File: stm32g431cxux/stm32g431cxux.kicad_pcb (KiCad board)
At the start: 2 copper layers, 17.8 x 31.2 mm, 23 parts, among them J1 USB2.0_C_v3, J2 ProMicro-LeftPin-NoGND, J3 ProMicro-RightPin, SW1 SW_Push, U1 AMS1117-3.3, U2 STM32G431CBUx, Y1 24M

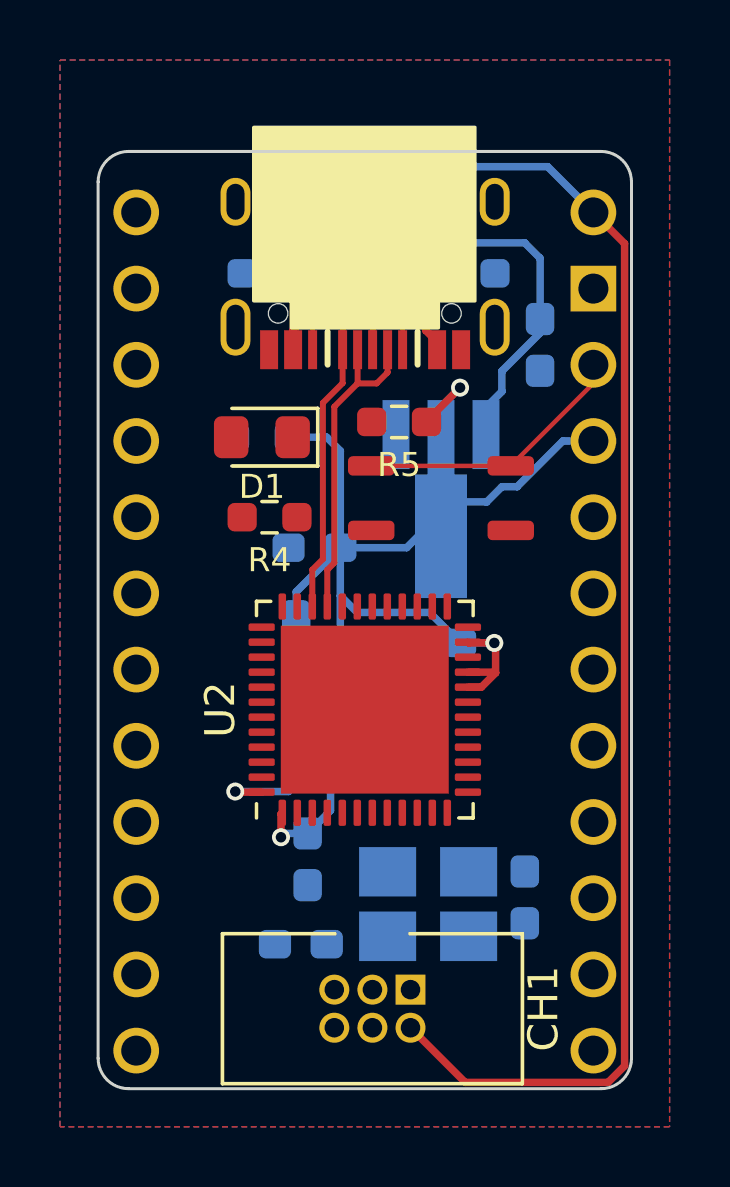
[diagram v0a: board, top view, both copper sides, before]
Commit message: before free routing
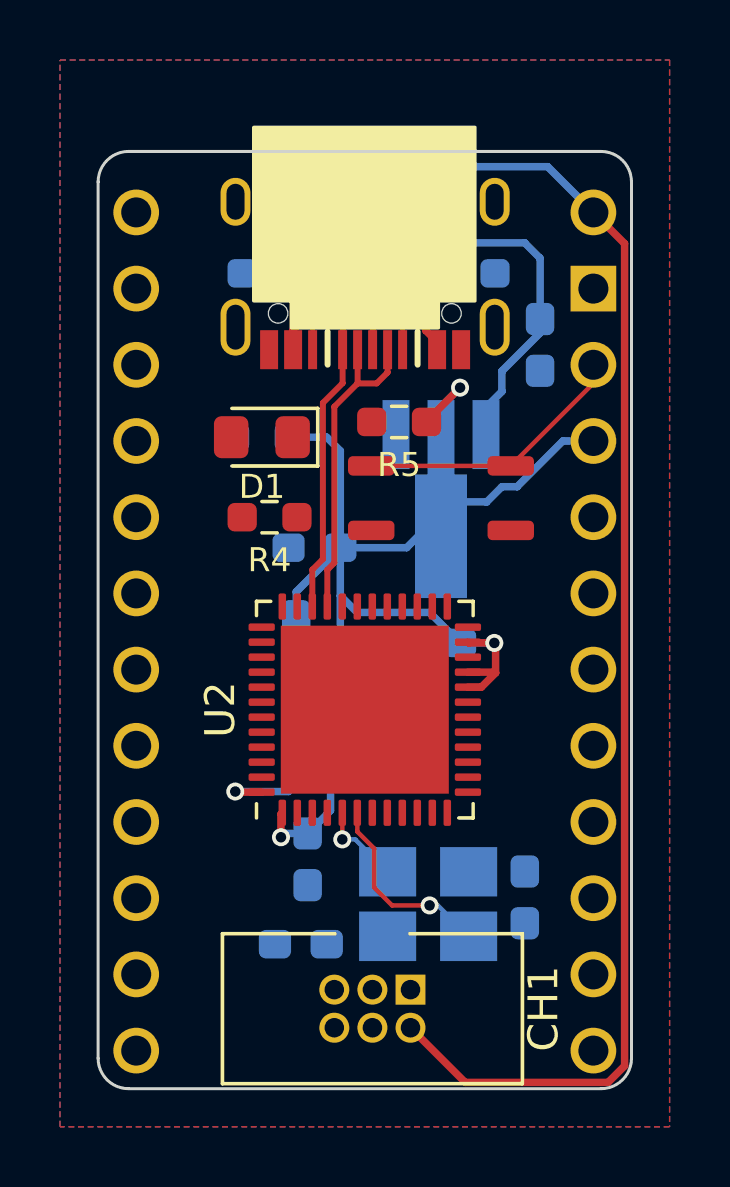
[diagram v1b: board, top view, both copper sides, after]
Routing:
- net Net-(U2-PF1): track 0.00 -> 6.55 mm, vias 0 -> 1
- net Net-(U2-PF0): track 0.00 -> 2.85 mm, vias 0 -> 1
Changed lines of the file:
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@@
   (segment (start 73.66 43.795) (end 73.66 43.18) (width 0.15) (layer "F.Cu") (net 30))
   (segment (start 66.255 46.55) (end 70.905 46.55) (width 0.15) (layer "F.Cu") (net 30))
+  (segment (start 65.29 59) (end 65.29 58.1125) (width 0.15) (layer "F.Cu") (net 35))
+  (via (at 65.29 59) (size 0.6) (drill 0.35) (layers "F.Cu" "B.Cu") (net 35))
+  (segment (start 65.722 59) (end 66.802 60.08) (width 0.15) (layer "B.Cu") (net 35))
+  (segment (start 65.29 59) (end 65.722 59) (width 0.15) (layer "B.Cu") (net 35))
+  (segment (start 65.79 58.74) (end 66.35 59.3) (width 0.15) (layer "F.Cu") (net 36))
+  (segment (start 65.79 58.1125) (end 65.79 58.74) (width 0.15) (layer "F.Cu") (net 36))
+  (segment (start 66.35 60.6) (end 66.95 61.2) (width 0.15) (layer "F.Cu") (net 36))
+  (segment (start 66.95 61.2) (end 68.2 61.2) (width 0.15) (layer "F.Cu") (net 36))
+  (segment (start 66.35 59.3) (end 66.35 60.6) (width 0.15) (layer "F.Cu") (net 36))
+  (via (at 68.2 61.2) (size 0.6) (drill 0.35) (layers "F.Cu" "B.Cu") (net 36))
+  (segment (start 68.472 61.2) (end 69.502 62.23) (width 0.15) (layer "B.Cu") (net 36))
+  (segment (start 68.2 61.2) (end 68.472 61.2) (width 0.15) (layer "B.Cu") (net 36))
   (zone (net 2) (net_name "GND") (layers "F&B.Cu") (hatch edge 0.5)
     (connect_pads (clearance 0.5))
